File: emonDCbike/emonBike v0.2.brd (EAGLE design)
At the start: 99.1 x 76.5 mm, 85 parts, among them Q1 16Mhz XT49M-2016M, U1_TQFP ATMEGA328P

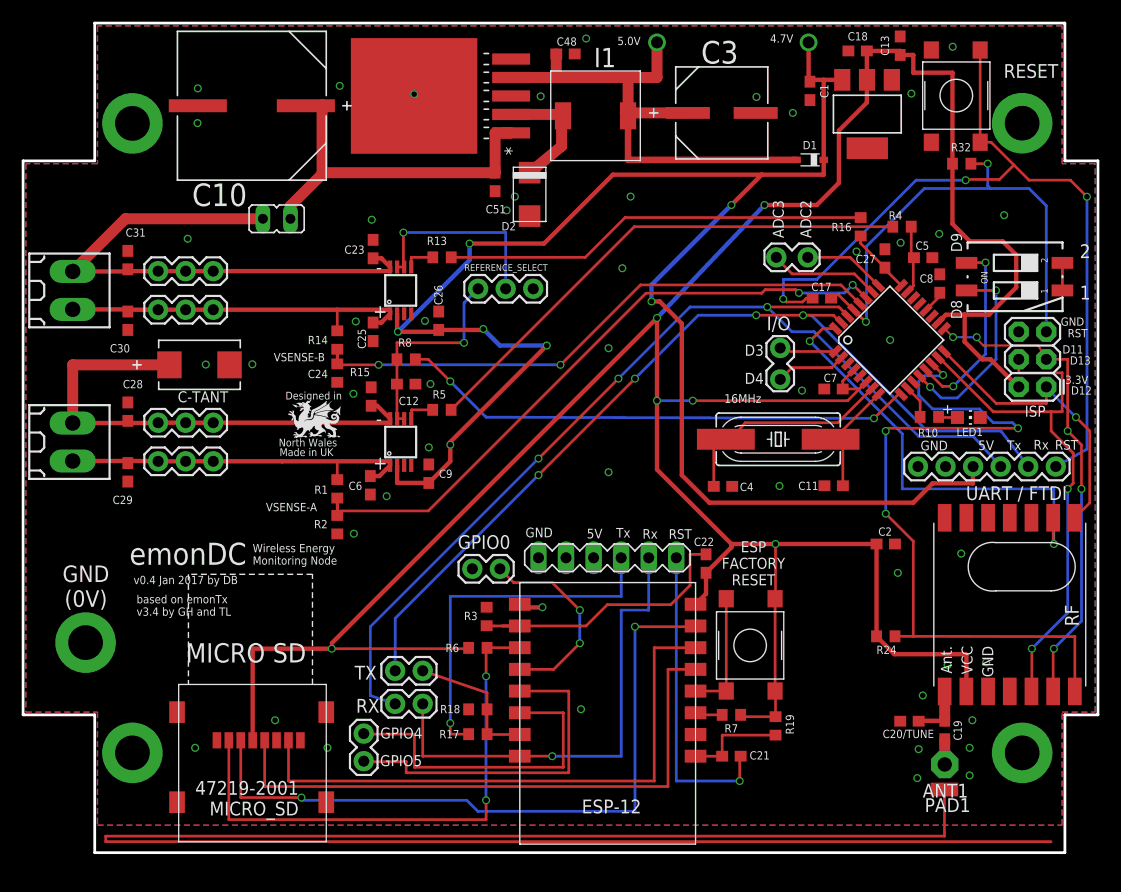
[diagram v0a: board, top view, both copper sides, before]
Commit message: updating v1.0
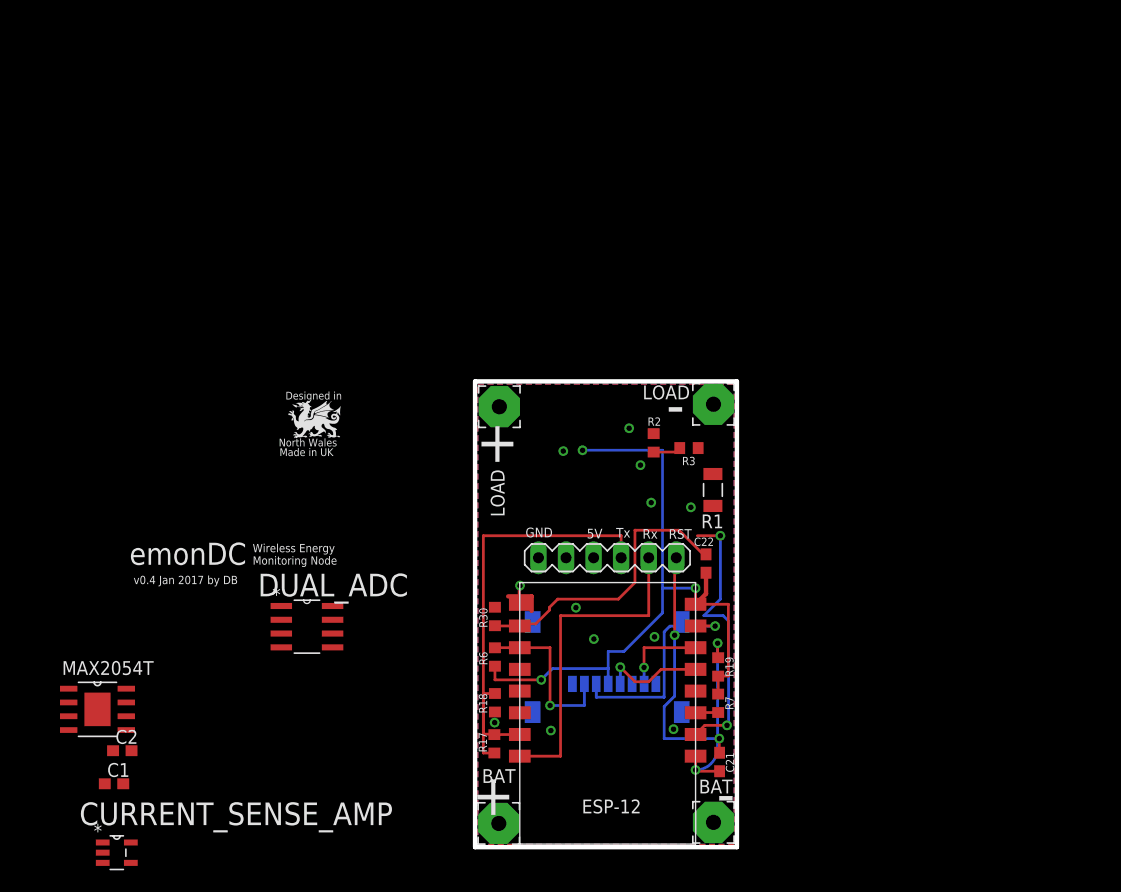
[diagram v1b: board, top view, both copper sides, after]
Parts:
- removed 3.3V_REG: REG1117, burr-brown:SOT223
- removed 5V_REG: TL2575HV, TL2575HV:TO-263
- removed ANA, I/O: 2212S-02SG-85, SparkFun-Connectors:1X02_LOCK
- removed ANT1: (no value), discrete:PAD-01
- removed C-TANT: 10uF 63V, 2917 footprint capacitor:2917
- removed C10: 100uF 80V, Panasonic-EEE-EEV-EEF-ECQ:CAPAE1350X1400N
- removed C11, C19, C4: 22pF, rcl:C0603
- removed C12: 220nF, rcl:C0603
- removed C13, C17, C27, C48, C5, C51, C7, C8: 100nF, rcl:C0603
- removed C18: 10uF TANT, rcl:C0603
- removed C20/TUNE: tune, rcl:C0603
- removed C23, C24, C25, C26, C28, C29, C30, C31, C6, C9: 0.1uF 100V, rcl:C0603
- removed C3: 470uF, Panasonic-EEEFK_EEEFP:CAPAE830X1050N
- removed D1: BAT60J, diode:SOD323_ST
- removed D2: MBRA130LT3G, CASE 403D Diode:DO-214
- removed FTDI/UART: 2211S-06G, SparkFun:FTDI_BASIC
- removed GPIO-4/5, GPIO0, RX, TX: (no value), SparkFun:1X02
- removed I1: 330uH, SRR0603-331KL:SRR0603-331KL
- removed ISP: M20-9980346, SparkFun:2X3
- removed J1, J2, J3, J4: (no value), SparkFun-Connectors:1X03
- removed JP3: 2211S-02G, jumper:JP1
- removed LED1: Red 1.85V, adafruit:CHIP-LED0805
- removed MC1, MC32882: MC32882, multicomp tact switch:SWITCH_TACT_MULTICOMP
- removed Q1: 16Mhz XT49M-2016M, adafruit:HC49UP
- removed R10, R13, R5: 1K, rcl:R0603
- removed R14: 100K 60V, rcl:R0603
- removed R15: 5.9K, rcl:R0603
- removed R16, R4: 9K1, rcl:R0603
- removed R24: 120K, rcl:R0603
- removed R32: 10K, rcl:R0603
- removed R8: 3.9K, rcl:R0603
- removed REFERENCE_SELECT: 2212S-02SG-85, SparkFun-Connectors:1X03
- removed RF: RFM12B, JeeParts:RFM12B
- removed S3: A6S-2104-PH, OpenEnergyMonitor:DIP_SWITCH_SMT
- removed SHUNTMON-A, SHUNTMON-B: LMP8481, lmp8481b:S-PDSO-G08
- removed T1, T2: (no value), con-weidmueller-sl35:180-2
- removed U1_TQFP: ATMEGA328P, SparkFun-DigitalIC:TQFP32-08
- added CURRENT_SENSE_AMP: ZXCT1086E5TA, Diodes_Inc-ZXCT1086E5TA:SOT95P280X130-5N
- added DUAL_ADC: MCP3002-I/SN, Microchip-MCP3002-I_SN:SOIC127P600X175-8N
- added PAD2, PAD3, PAD4: (no value), wirepad:3,81/1,4
- added R30: 10k, rcl:R0603
- added U1YEAH: MAX5023TASA-T, MAX2053:21-0111D_SBE-14
- C2: value 100nF -> 10uF TANT
- PAD1: device wirepad:SMD1,27-2,54 -> wirepad:3,81/1,4
- R1: value 100K 60V -> 0.022 OHM; device rcl:R0603 -> Panasonic-ERJ3_ERJ8_ERJA_ERJB:RESC3216X71N
- R2: value 5.9K -> 100K 60V
- R3: value 10k -> 5.9K
- moved C1 90.5 mm to (8.64, 8.13), turned to 0 degrees
- moved C2 72.9 mm to (9.40, 11.2)
- moved PAD1 41.2 mm to (44.1, 4.47), turned to 0 degrees
- moved R1 34.6 mm to (63.8, 35.2)
- moved U$1 32.8 mm to (61.0, 14.7), flipped to the bottom, turned to 0 degrees
- moved R2 30.1 mm to (58.4, 39.5)
- moved R3 24.3 mm to (61.6, 39.1), turned to 180 degrees
- moved R19 7.58 mm to (64.3, 18.9), turned to 270 degrees
- moved R6 1.78 mm to (43.7, 19.8), turned to 270 degrees
- moved R17 1.76 mm to (43.7, 11.8), turned to 90 degrees
- moved R18 1.69 mm to (43.7, 15.6), turned to 270 degrees
- moved R7 1.62 mm to (64.3, 15.5), turned to 90 degrees
- moved C21 1.22 mm to (64.4, 10.1), turned to 90 degrees
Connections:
- removed net 4.7V: 3.3V_REG.3, C1.1, C26.1, C9.1, D1.C, FTDI/UART.VCC, SHUNTMON-A.2, SHUNTMON-B.2
- removed net 5.0V: 5V_REG.4, C3.1, C48.1, D1.A, I1.P$2
- removed net ADC2: ANA.1, U1_TQFP.25
- removed net ADC3: ANA.2, U1_TQFP.26
- removed net ADCSHUNT-A: R13.2, R16.2
- removed net ADCSHUNT-B: R4.2, R5.2
- removed net ADCVSENSE-B: R1.1, R2.2, U1_TQFP.27
- removed net AGND: U1_TQFP.21
- removed net D0/RX: FTDI/UART.TXO, RX.2, U1_TQFP.30
- removed net D1/TX: FTDI/UART.RXI, TX.2, U1_TQFP.31
- removed net D10: R24.1, RF.SEL, U1_TQFP.14
- removed net D11/MOSI: ISP.4, RF.SDI, U1_TQFP.15
- removed net D12/MISO: ISP.1, RF.SDO, U1_TQFP.16
- removed net D13/SCK: ISP.3, RF.SCK, U1_TQFP.17
- removed net D2: RF.IRQ, U1_TQFP.32
- removed net D3: I/O.1, U1_TQFP.1
- removed net D4: I/O.2, U1_TQFP.2
- removed net D5/PWM0: R8.2, U1_TQFP.9
- removed net D6: R10.2, U1_TQFP.10
- removed net D7: U1_TQFP.11
- removed net D8: S3.4, U1_TQFP.12
- removed net D9: S3.3, U1_TQFP.13
- removed net DIG1: C19.1, C20/TUNE.1, RF.ANT
- removed net IND: 5V_REG.2, D2.P$1, I1.P$1
- removed net INPUT-POS-A: C25.1, C30.1, J2.1, J2.2, J2.3, R14.2, SHUNTMON-A.1, T1.2
- removed net INPUT-POS-B: C29.1, C6.1, J3.1, J3.2, J3.3, R1.2, SHUNTMON-B.1, T2.2
- removed net LOAD-NEG-A: C23.2, C31.1, J1.1, J1.2, J1.3, JP3.2, SHUNTMON-A.8, T1.1
- removed net LOAD-NEG-B: C-TANT.1, C24.2, C28.1, J4.1, J4.2, J4.3, SHUNTMON-B.8, T2.1
- removed net N$1: C4.1, Q1.2, U1_TQFP.7
- removed net N$20: C8.1, U1_TQFP.20
- removed net N$27: C27.2, R16.1, U1_TQFP.24
- removed net N$28: REFERENCE_SELECT.2, SHUNTMON-A.6, SHUNTMON-A.7
- removed net N$4: R13.1, SHUNTMON-A.5
- removed net N$41: LED1.A, R10.1
- removed net N$5: PAD1.1
- removed net N$6: R5.1, SHUNTMON-B.5
- removed net N$9: C11.1, Q1.1, U1_TQFP.8
- removed net POWERIN: 5V_REG.1, C10.1, C51.1, JP3.1
- removed net REFINPUT: C12.1, R8.1, REFERENCE_SELECT.1, SHUNTMON-B.6, SHUNTMON-B.7
- removed net RES: C17.1, FTDI/UART.DTR, MC32882.P$1, MC32882.P$2
- removed net RESET: C17.2, ISP.5, R32.1, U1_TQFP.29
- new net INPUT-POS: C2.1, U1YEAH.1
- new net VDD/VREF: DUAL_ADC.8
- new net VSS: DUAL_ADC.4
- net 3.3V: now also C1.1, U1YEAH.8; no longer 3.3V_REG.2, C13.1, C18.1, C2.1, C7.1, ISP.2, MC1.P$3, MC1.P$4, R24.2, R32.2, RF.VDD, U1_TQFP.18, U1_TQFP.4, U1_TQFP.6
- net ADCVSENSE-A: now also R2.1, R3.2; no longer R14.1, R15.2, U1_TQFP.28
- net ESPRX: no longer TX.1
- net ESPTX: no longer RX.1
- net GND: now also CURRENT_SENSE_AMP.2, PAD3.1, PAD4.1, R30.1, U1YEAH.3; no longer 3.3V_REG.1, 5V_REG.3, 5V_REG.5, 5V_REG.6, C-TANT.2, C10.2, C11.2, C12.2, C13.2, C18.2, C20/TUNE.2, C23.1, C24.1, C25.2, C26.2, C27.1, C28.2, C29.2, C3.2, C30.2, C31.2, C4.2, C48.2, C5.1, C51.2, C6.2, C7.2, C8.2, C9.2, D2.P$2, FTDI/UART.GND, GPIO0.1, ISP.6, LED1.C, MC32882.P$3, MC32882.P$4, R15.1, R2.1, REFERENCE_SELECT.3, RF.GND, RF.P$12, S3.1, S3.2, SHUNTMON-A.4, SHUNTMON-B.4, U1_TQFP.3, U1_TQFP.5
- net GPIO0: no longer GPIO0.2
- net GPIO15: now also R30.2; no longer R3.2
- net GPIO16: no longer MC1.P$1, MC1.P$2
- net GPIO4: no longer GPIO-4/5.1
- net GPIO5: no longer GPIO-4/5.2
- net N$2: now also CURRENT_SENSE_AMP.4, PAD1.1, R1.1; no longer C5.2, R4.1, U1_TQFP.23
- net N$3: now also CURRENT_SENSE_AMP.3, CURRENT_SENSE_AMP.5, PAD2.1, R1.2, R2.2; no longer ANT1.1, C19.2
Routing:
- net 3.3V: track 267.5 -> 64.0 mm, vias 6 -> 3
- net N$31: track 168.7 -> 0.00 mm
- net 4.7V: track 163.5 -> 0.00 mm, vias 8 -> 0
- net D0/RX: track 93.0 -> 0.00 mm, vias 3 -> 0
- net D1/TX: track 84.6 -> 0.00 mm, vias 4 -> 0
- net RES: track 77.6 -> 0.00 mm, vias 3 -> 0
- net D10: track 69.7 -> 0.00 mm, vias 4 -> 0
- net ADCVSENSE-B: track 60.9 -> 0.00 mm, vias 2 -> 0
- net ADCVSENSE-A: track 54.7 -> 2.55 mm, vias 2 -> 0
- net LOAD-NEG-A: track 51.2 -> 0.00 mm
- net D11/MOSI: track 50.6 -> 0.00 mm, vias 2 -> 0
- net LOAD-NEG-B: track 48.4 -> 0.00 mm
- net 5.0V: track 48.1 -> 0.00 mm, vias 1 -> 0
- net D5/PWM0: track 48.0 -> 0.00 mm, vias 2 -> 0
- net ADCSHUNT-B: track 47.7 -> 0.00 mm
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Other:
- board size 99.1 x 76.5 mm -> 24.1 x 42.9 mm
- board text added: "+"
- board text added: "-"
- board text added: "BAT"
- board text added: "LOAD"
- board text removed: "16MHz"
- board text removed: "2 1"
- board text removed: "3.3V"
- board text removed: "4.7V"
- board text removed: "5.0V"
- board text removed: "A"
- board text removed: "ADC2"
- board text removed: "ADC3"
- board text removed: "B"
- board text removed: "D11"
- board text removed: "D12"
- board text removed: "D13"
- board text removed: "D2"
- board text removed: "D3"
- board text removed: "D4"
- board text removed: "D8"
- board text removed: "D9"
- board text removed: "Designed in North Wales UK by Megni"
- board text removed: "ESP FACTORY RESET"
- board text removed: "GND (0V)"
- board text removed: "GPIO4"
- board text removed: "GPIO5"
- board text removed: "I1"
- board text removed: "MICRO SD"
- board text removed: "Node:"
- board text removed: "OpenEnergyMonitor.org"
- board text removed: "RESET"
- board text removed: "UART / FTDI"
- board text removed: "VSENSE-A"
- board text removed: "VSENSE-B"
- board text removed: "based on emonTx v3.4 by GH and TL"

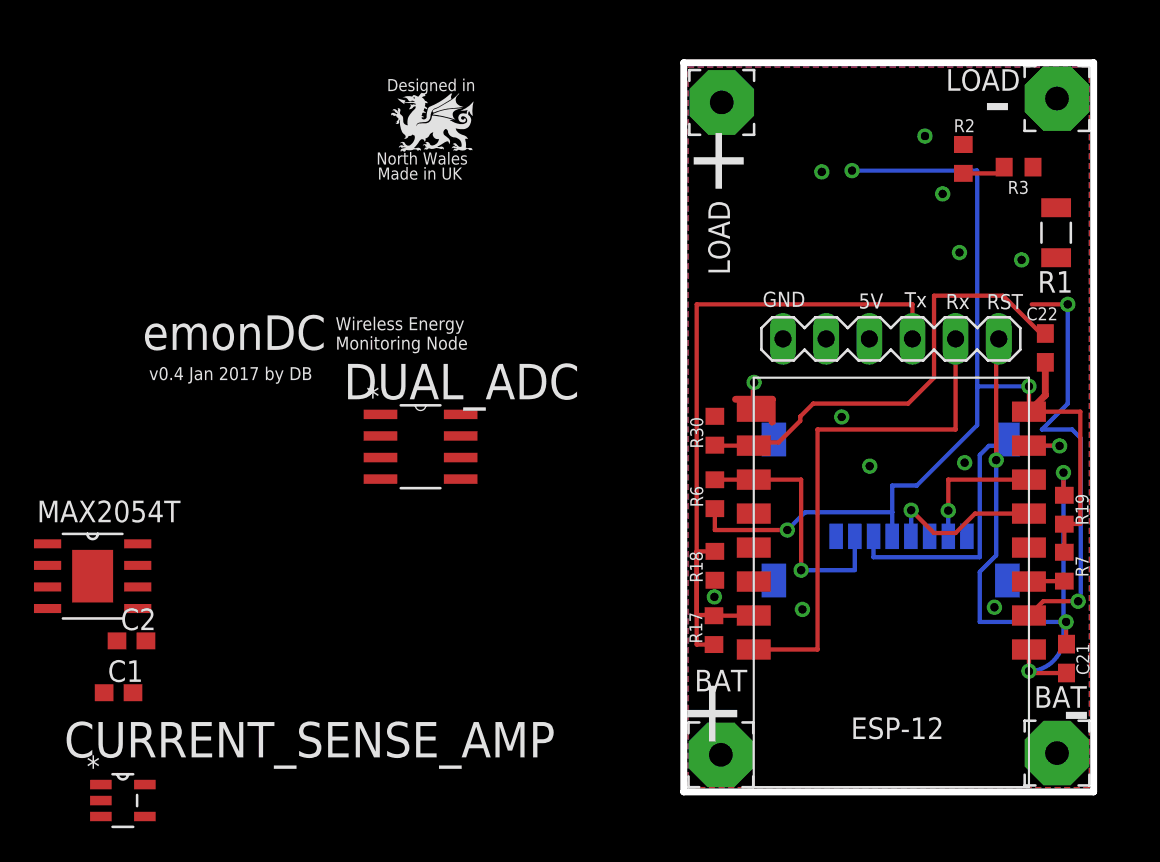
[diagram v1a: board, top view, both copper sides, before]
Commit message: emonBIKE v0.2 camexport
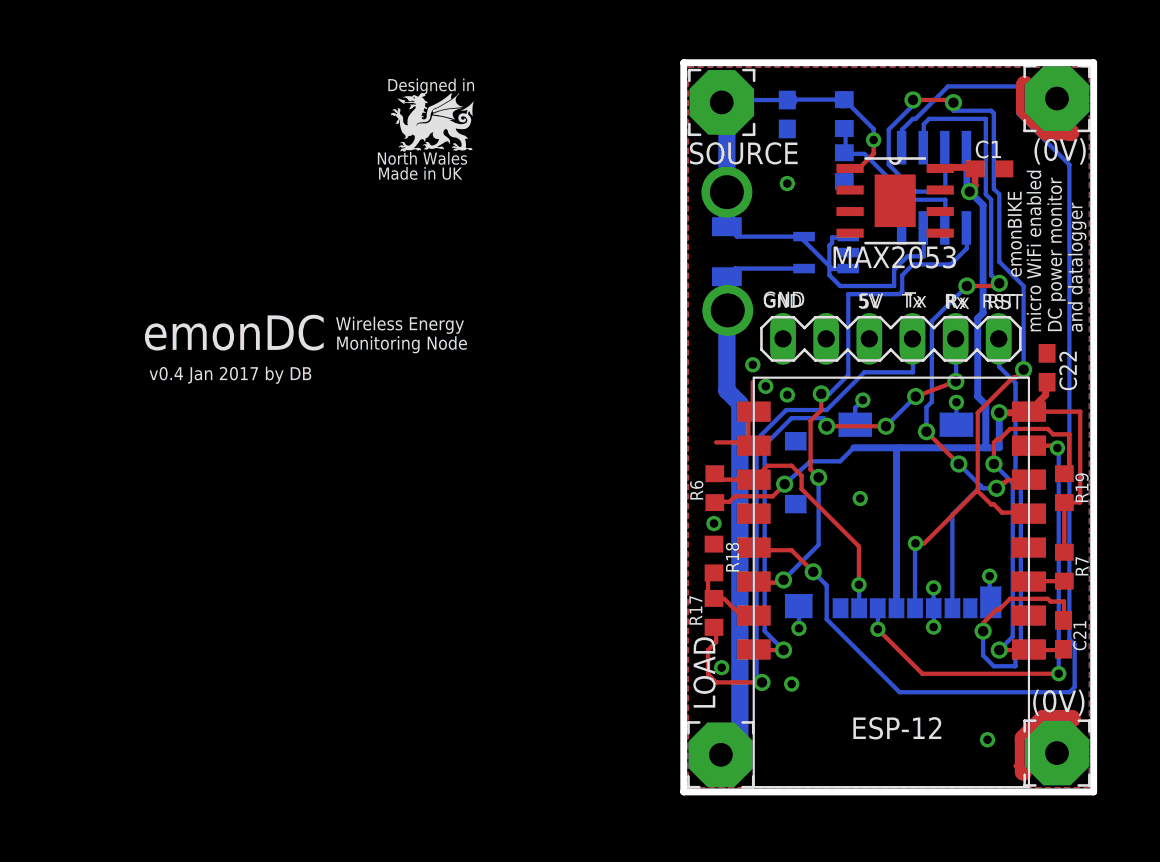
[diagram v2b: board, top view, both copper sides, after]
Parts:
- removed CURRENT_SENSE_AMP: ZXCT1086E5TA, Diodes_Inc-ZXCT1086E5TA:SOT95P280X130-5N
- removed DUAL_ADC: MCP3002-I/SN, Microchip-MCP3002-I_SN:SOIC127P600X175-8N
- removed R1: 0.022 OHM, Panasonic-ERJ3_ERJ8_ERJA_ERJB:RESC3216X71N
- removed R30: 10k, rcl:R0603
- removed U$1: 47219-2001_MICROSD, 47219-2001_SD_MICRO:47219-2001_MICROSD
- removed U1YEAH: MAX5023TASA-T, MAX2053:21-0111D_SBE-14
- added MAX2053: MAX5023TASA-T, MAX2053:21-0111D_SBE-14
- added MCP3002: MCP3002-I/SN, Microchip-MCP3002-I_SN:SOIC127P600X175-8N
- added R_SENSE: 0.022 OHM, Panasonic-ERJ3_ERJ8_ERJA_ERJB:RESC3216X71N
- added U$2: MOLEX_MICRO_SD_1040310811, MOLEX MICRO SD [exposed pins]:MOLEX_MICROSD_EXPOSED
- added U$3: (no value), DRAGON_LOGO:DRAGON_LOGO_NOTEXT
- added ZXCT1086: ZXCT1086E5TA, Diodes_Inc-ZXCT1086E5TA:SOT95P280X130-5N
- C1: value 10uF TANT -> 10uF 16V TANT
- C2: value 10uF TANT -> 10uF 60V TANT
- moved C1 59.8 mm to (59.9, 39.0)
- moved C2 49.5 mm to (48.0, 42.2), flipped to the bottom, turned to 270 degrees
- moved LOGO1 33.4 mm to (55.4, 5.36)
- moved R3 10.3 mm to (51.4, 39.1), flipped to the bottom, turned to 90 degrees
- moved R2 7.49 mm to (51.4, 42.2), flipped to the bottom
- moved C21 1.41 mm to (64.3, 11.5)
- moved R19 1.27 mm to (64.3, 20.2)
- moved C22 1.17 mm to (63.3, 27.3)
- moved R17 1.02 mm to (43.7, 12.8)
- moved R18 0.43 mm to (43.7, 16.0), turned to 90 degrees
- moved R6 0.36 mm to (43.7, 20.2)
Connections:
- removed net 3.3V: C1.1, C22.2, ESP-12.16, R19.2, R6.2, R7.2, U$1.PIN4, U1YEAH.8
- removed net ADCVSENSE-A: R2.1, R3.2
- removed net GPIO15: C22.1, ESP-12.1, ESP-12.2, R30.2
- removed net INPUT-POS: C2.1, U1YEAH.1
- removed net N$2: CURRENT_SENSE_AMP.4, PAD1.1, R1.1
- removed net N$3: CURRENT_SENSE_AMP.3, CURRENT_SENSE_AMP.5, PAD2.1, R1.2, R2.2
- removed net N$32: U$1.PIN8
- removed net N$7: U$1.PIN1
- removed net VDD/VREF: DUAL_ADC.8
- removed net VSS: DUAL_ADC.4
- new net +3V3: C1.1, C22.2, ESP-12.16, MAX2053.8, MCP3002.8, R19.2, R6.2, R7.2, U$2.P$4
- new net ADC_CSENSE: MCP3002.3, ZXCT1086.1
- new net ADC_VSENSE: MCP3002.2, R2.1, R3.2
- new net LOAD-: PAD1.1, R_SENSE.1, ZXCT1086.4
- new net SOURCE+: C2.1, MAX2053.1, PAD2.1, R2.2, R_SENSE.2, ZXCT1086.3, ZXCT1086.5
- net GND: now also C22.1, ESP-12.1, ESP-12.2, MAX2053.3, MCP3002.4, U$2.GND1, U$2.GND2, U$2.GND3, U$2.GND4, U$2.P$6, ZXCT1086.2; no longer CURRENT_SENSE_AMP.2, R30.1, U$1.P$1, U$1.P$2, U$1.P$3, U$1.P$4, U$1.PIN6, U1YEAH.3
- net GPIO12: now also MCP3002.6, U$2.P$7; no longer U$1.PIN7
- net GPIO13: now also U$2.P$3; no longer U$1.PIN3
- net GPIO14: now also MCP3002.7, U$2.P$5; no longer U$1.PIN5
- net GPIO2: now also U$2.P$2; no longer U$1.PIN2
- net GPIO4: now also MCP3002.1
- net GPIO5: now also MCP3002.5
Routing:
- net GPIO5: track 0.00 -> 69.4 mm, vias 0 -> 1
- net +3V3: track 0.00 -> 68.5 mm, vias 0 -> 3
- net 3.3V: track 64.0 -> 0.00 mm, vias 3 -> 0
- net GPIO14: track 9.51 -> 52.9 mm, vias 1 -> 4
- net GPIO12: track 8.09 -> 42.2 mm, vias 1 -> 5
- net LOAD-: track 0.00 -> 33.9 mm
- net GPIO4: track 0.00 -> 30.8 mm, vias 0 -> 3
- net SOURCE+: track 0.00 -> 28.6 mm, vias 0 -> 1
- net GPIO15: track 27.0 -> 0.00 mm
- net ADC: track 25.5 -> 0.00 mm, vias 2 -> 0
- net GND: track 5.28 -> 25.5 mm, vias 12 -> 15
- net ADC_CSENSE: track 0.00 -> 12.0 mm
- net ADC_VSENSE: track 0.00 -> 10.3 mm
- net GPIO13: track 20.2 -> 28.2 mm, vias 1 -> 3
- net N$30: track 23.6 -> 30.6 mm, vias 2 -> 1
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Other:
- board text added: "(0V)"
- board text added: "SOURCE"
- board text added: "emonBIKE"
- board text added: "micro WiFi enabled DC power monitor and datalogger"
- board text removed: "+"
- board text removed: "-"
- board text removed: "BAT"
- board text removed: "Lead free PCB - RoHS components"
